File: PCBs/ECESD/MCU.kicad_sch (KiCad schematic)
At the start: 16 parts, among them J200 1332645, SW200 SW_Omron_B3FS, SW201 SW_Omron_B3FS, U200 ESP32-C3-MINI-1-N4, U201 USBLC6-2SC6

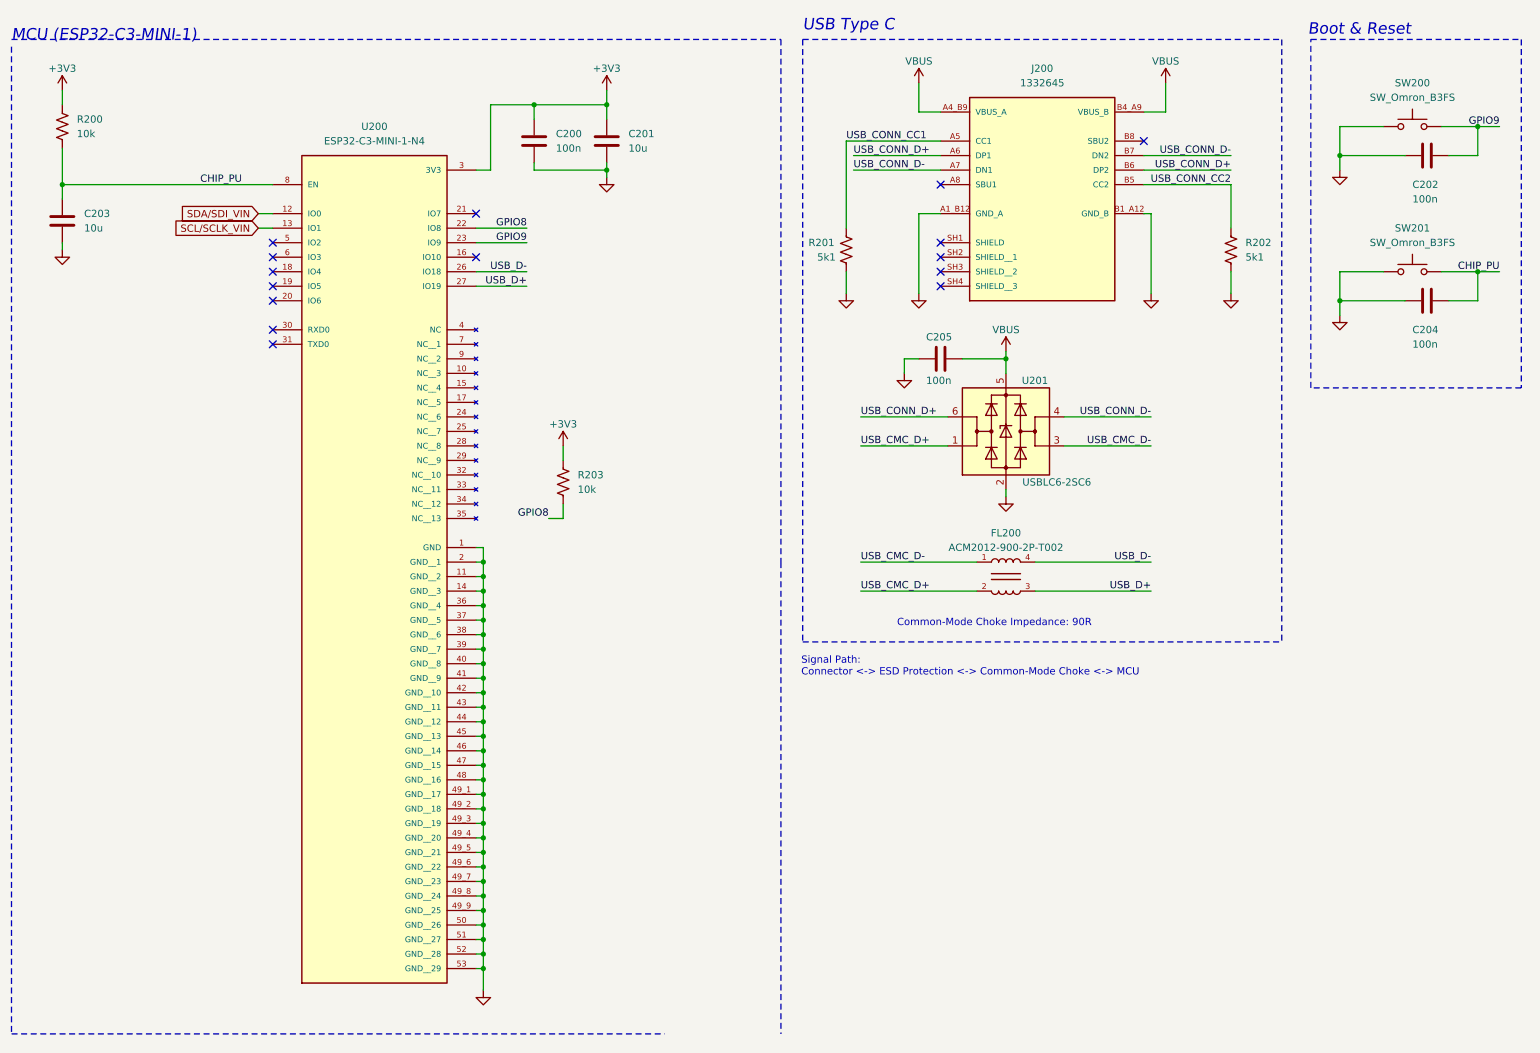
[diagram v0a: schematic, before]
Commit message: Changed PCB 1
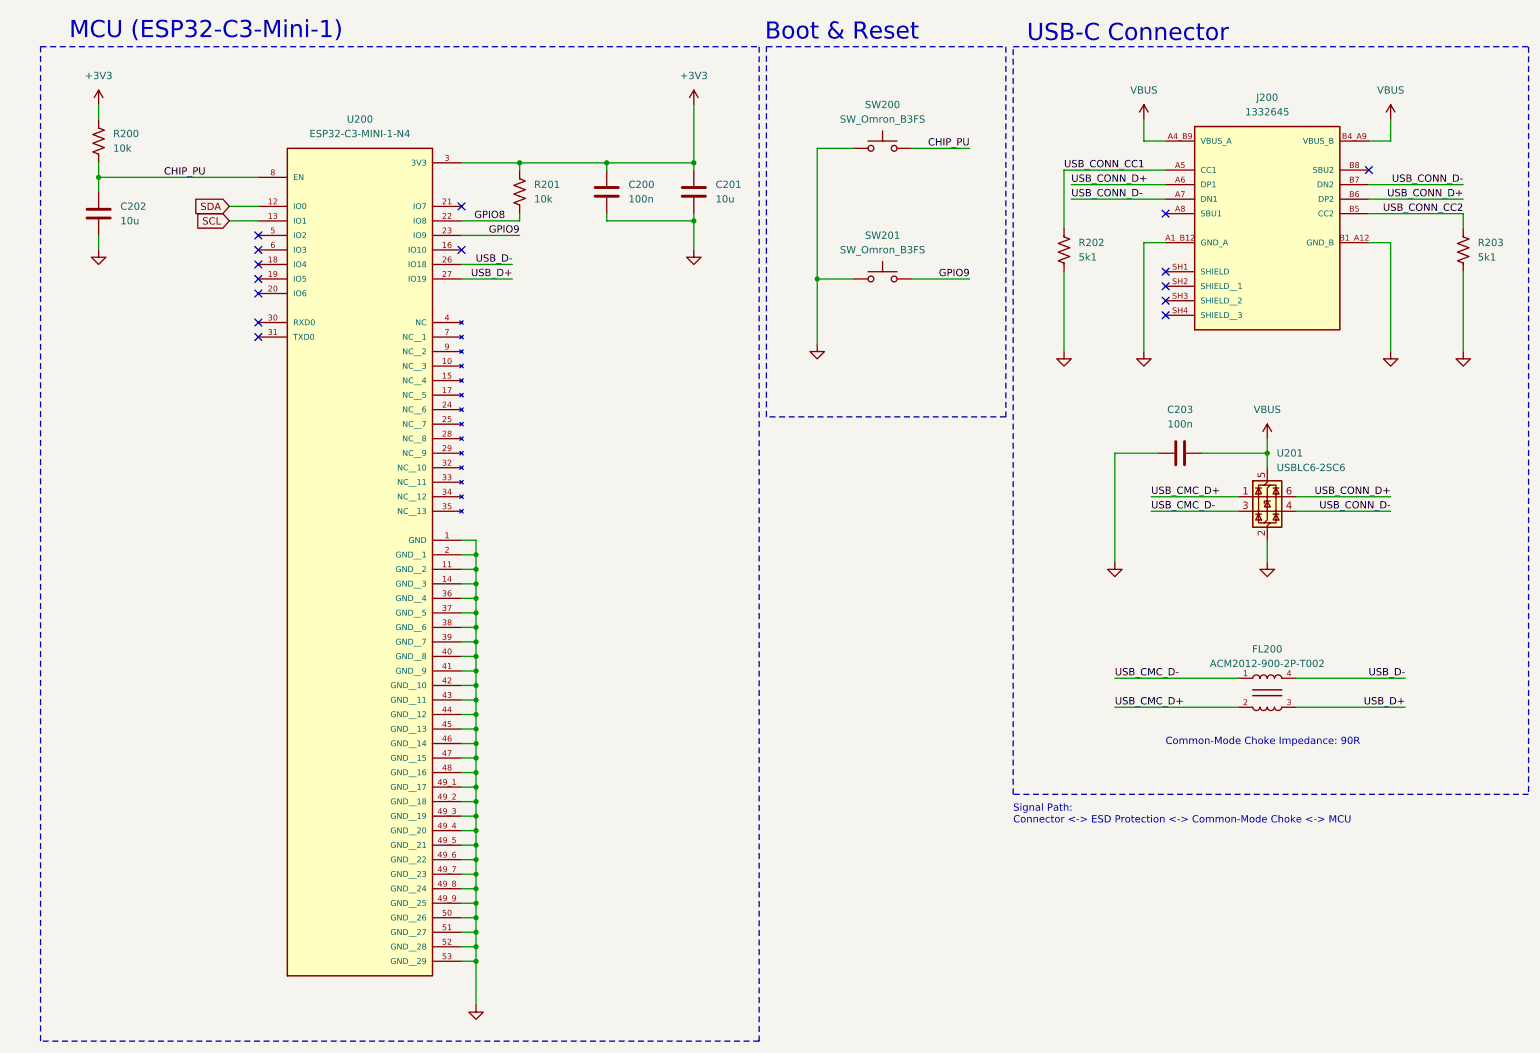
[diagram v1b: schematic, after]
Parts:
- removed C204, C205: 100n, Capacitor_SMD:C_0603_1608Metric_Pad1.08x0.95mm_HandSolder, symbol Device:C
- removed FL200: ACM2012-900-2P-T002, ACM2012_900_2P_T002:FIL_ACM2012-900-2P-T002, symbol ACM2012-900-2P-T002:ACM2012-900-2P-T002
- removed U201: USBLC6-2SC6, Package_TO_SOT_SMD:SOT-23-6, symbol Nemesis-MixSigPCB-rescue:USBLC6-2SC6-Power_Protection
- added FL200: ACM2012-900-2P-T002, CMC:FIL_ACM2012-900-2P-T002, symbol CMC:ACM2012-900-2P-T002
- added U201: USBLC6-2SC6, Package_TO_SOT_SMD:SOT-23-6, symbol Power_Protection:USBLC6-2SC6
- C202: value 100n -> 10u
- C203: value 10u -> 100n
- R201: value 5k1 -> 10k
- R203: value 10k -> 5k1
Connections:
- net +3V3: now also R201.1; no longer R203.1
- net CHIP_PU: now also C202.1, SW200.2; no longer C203.1, SW201.2
- net GND: now also R203.2, U201.2 (GND); no longer R201.2
- net GPIO8: now also R201.2; no longer R203.2
- net GPIO9: now also SW201.2; no longer C202.1, SW200.2
- net USB_CMC_D+: now also FL200.2, U201.1 (I/O1)
- net USB_CMC_D-: now also FL200.1, U201.3 (I/O2)
- net USB_CONN_CC1: now also R202.1; no longer R201.1
- net USB_CONN_CC2: now also R203.1; no longer R202.1
- net USB_CONN_D+: now also U201.6 (I/O1)
- net USB_CONN_D-: now also U201.4 (I/O2)
- net USB_D+: now also FL200.3
- net USB_D-: now also FL200.4
- net VBUS: now also C203.1, U201.5 (VBUS)
- net SCL/SCLK_VIN renamed SCL
- net SDA/SDI_VIN renamed SDA
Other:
- note added: "MCU (ESP32-C3-Mini-1)"
- note added: "USB-C Connector"
- note removed: "MCU (ESP32-C3-MINI-1)"
- note removed: "USB Type C"
